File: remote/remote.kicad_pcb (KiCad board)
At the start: 2 copper layers, 0 parts

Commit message: devlog 04
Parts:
- added C1: 100nF, Capacitor_SMD:C_0603_1608Metric, F.Cu at (0.00, 0.00)
- added C2: 10uF, Capacitor_SMD:C_0603_1608Metric, F.Cu at (0.00, 0.00)
- added C3: 1uF, Capacitor_SMD:C_0603_1608Metric, F.Cu at (0.00, 0.00)
- added D_CHG: CHG, LED_SMD:LED_0603_1608Metric, F.Cu at (0.00, 0.00)
- added D_STAT: STATUS, LED_SMD:LED_0603_1608Metric, F.Cu at (0.00, 0.00)
- added D_VBAT, D_VBUS: SS14, Diode_SMD:D_SMA, F.Cu at (0.00, 0.00)
- added HDR1: DEBUG, Connector_PinHeader_2.54mm:PinHeader_1x03_P2.54mm_Vertical, F.Cu at (0.00, 0.00)
- added J1: USB-C, Connector_USB:USB_C_Receptacle_HRO_TYPE-C-31-M-12, F.Cu at (0.00, 0.00)
- added J_BAT: BAT, Connector_JST:JST_PH_B2B-PH-K_1x02_P2.00mm_Vertical, F.Cu at (0.00, 0.00)
- added R_CC1, R_CC2: 5.1k, Resistor_SMD:R_0603_1608Metric, F.Cu at (0.00, 0.00)
- added R_CHG, R_STAT: 1k, Resistor_SMD:R_0603_1608Metric, F.Cu at (0.00, 0.00)
- added R_DN, R_UP: 100k, Resistor_SMD:R_0603_1608Metric, F.Cu at (0.00, 0.00)
- added R_EN: 10k, Resistor_SMD:R_0603_1608Metric, F.Cu at (0.00, 0.00)
- added R_PROG: 2k, Resistor_SMD:R_0603_1608Metric, F.Cu at (0.00, 0.00)
- added SW1: Choc1, clicker:Choc_V1_PG1350, F.Cu at (0.00, 0.00)
- added SW2: Choc2, clicker:Choc_V1_PG1350, F.Cu at (0.00, 0.00)
- added SW_BOOT: BOOT, Button_Switch_SMD:SW_SPST_B3U-1000P, F.Cu at (0.00, 0.00)
- added SW_PWR: POWER, Button_Switch_THT:SW_Slide_SPDT_Straight_CK_OS102011MS2Q, F.Cu at (0.00, 0.00)
- added SW_RST: RESET, Button_Switch_SMD:SW_SPST_B3U-1000P, F.Cu at (0.00, 0.00)
- added U1: ESP32-C3-WROOM-02, RF_Module:ESP32-C3-WROOM-02, F.Cu at (0.00, 0.00)
- added U2: MCP73831, Package_TO_SOT_SMD:SOT-23-5, F.Cu at (0.00, 0.00)
- added U3: AP2112K-3.3, Package_TO_SOT_SMD:SOT-23-5, F.Cu at (0.00, 0.00)

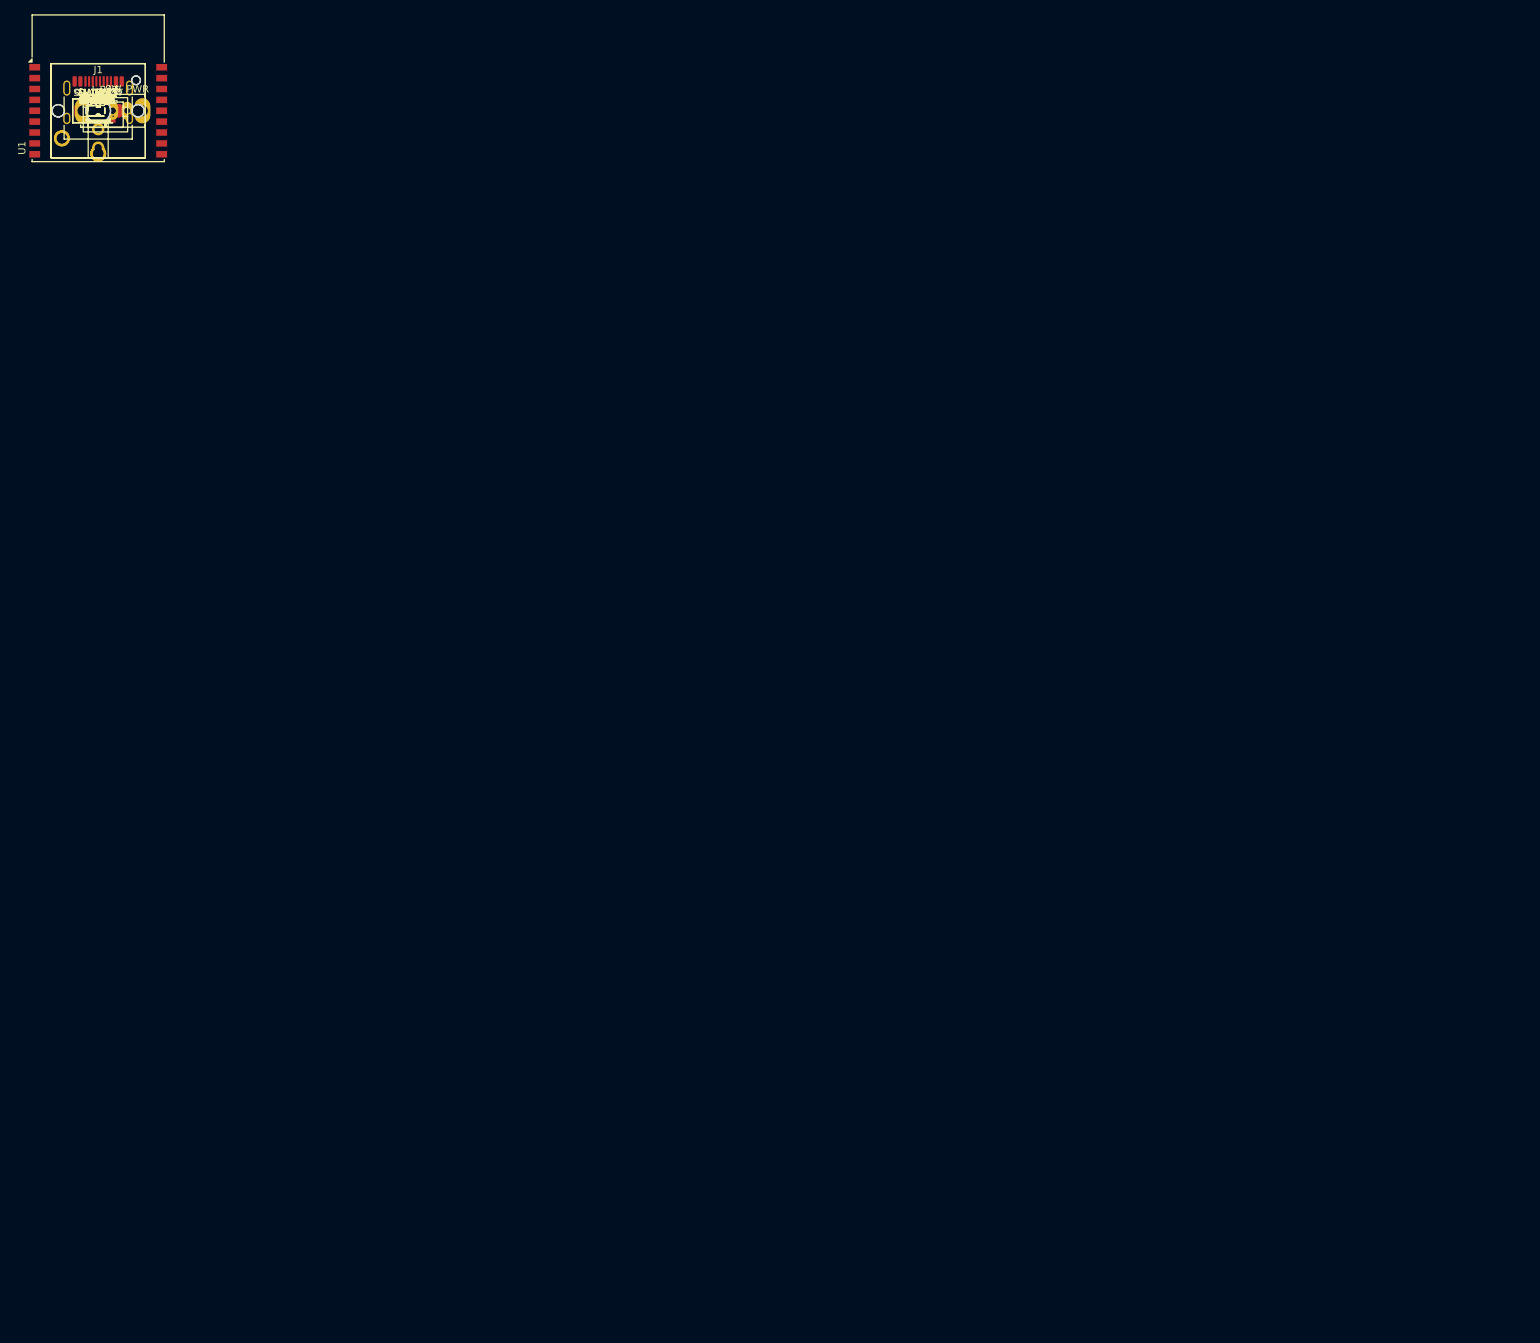
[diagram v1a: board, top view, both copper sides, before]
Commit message: devlog 06
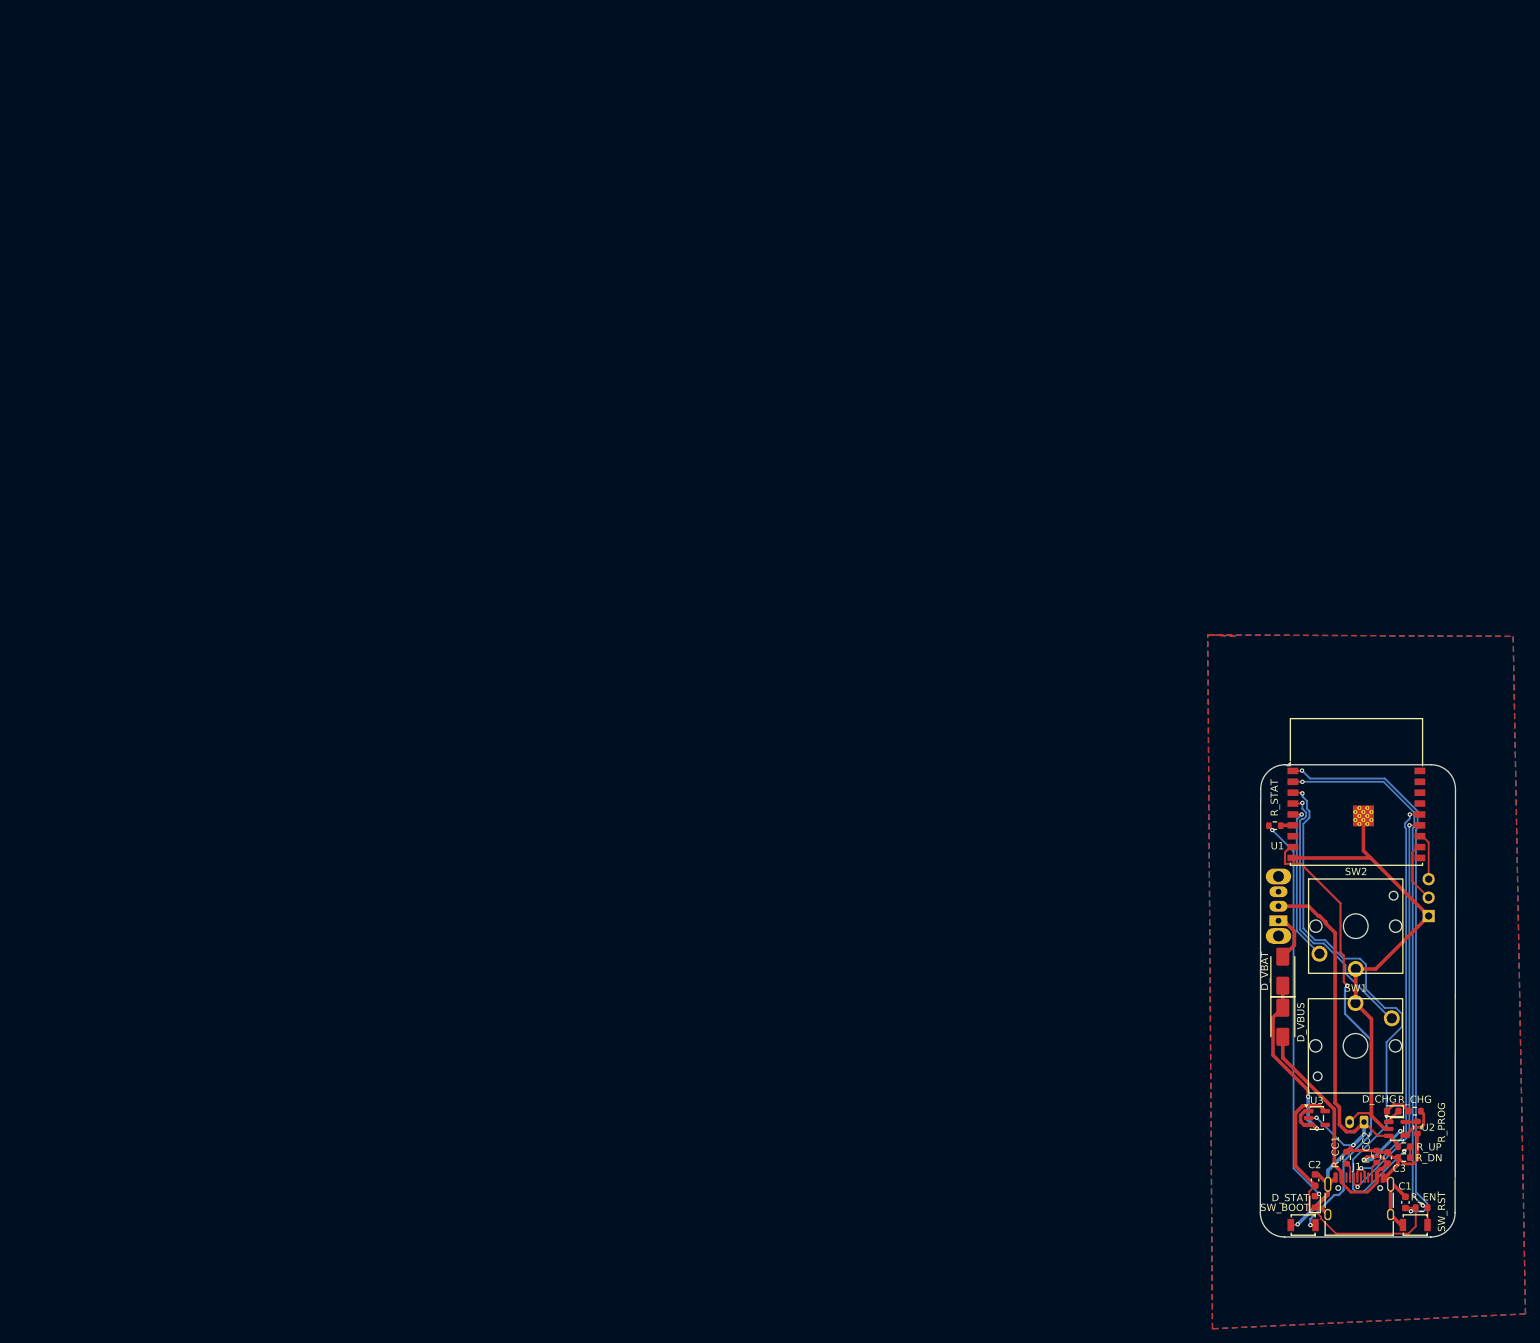
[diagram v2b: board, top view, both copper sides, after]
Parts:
- HDR1, J_BAT, SW_PWR: moved to B.Cu
- moved SW_RST 237.8 mm to (181.6, 153.6)
- moved R_EN 237.0 mm to (182.4, 151.2), turned to 180 degrees
- moved C1 234.8 mm to (180.2, 150.5), turned to 90 degrees
- moved R_DN 230.7 mm to (180.0, 144.3), turned to 180 degrees
- moved J1 230.3 mm to (173.8, 151.1)
- moved R_UP 229.8 mm to (180.0, 142.8)
- moved R_PROG 229.6 mm to (181.8, 140.2), turned to -90 degrees
- moved C3 229.0 mm to (177.8, 144.3), turned to 90 degrees
- moved R_CHG 227.9 mm to (181.5, 137.9), turned to 180 degrees
- moved R_CC2 227.7 mm to (176.2, 144.2), turned to 90 degrees
- moved U2 227.5 mm to (179.0, 140.3)
- moved SW_BOOT 226.2 mm to (166.1, 153.6)
- moved D_CHG 225.5 mm to (178.4, 137.9), turned to 180 degrees
- moved D_STAT 225.3 mm to (167.8, 150.4), turned to 90 degrees
- moved R_CC1 224.6 mm to (172.1, 144.3), turned to 90 degrees
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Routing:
- net GND: track 0.00 -> 136.1 mm, vias 0 -> 3
- net 3v3: track 0.00 -> 118.5 mm, vias 0 -> 2
- net VSENSE: track 0.00 -> 80.2 mm, vias 0 -> 2
- net EN_NET: track 0.00 -> 76.5 mm, vias 0 -> 2
- net BOOT_NET: track 0.00 -> 63.8 mm, vias 0 -> 2
- net USB_DN: track 0.00 -> 57.3 mm, vias 0 -> 2
- net USB_DP: track 0.00 -> 57.0 mm, vias 0 -> 2
- net STAT_A: track 0.00 -> 54.3 mm, vias 0 -> 2
- net VBUS: track 0.00 -> 49.6 mm, vias 0 -> 2
- net BAT_P: track 0.00 -> 46.7 mm
- net SW1_NET: track 0.00 -> 37.9 mm, vias 0 -> 1
- net VSYS: track 0.00 -> 27.7 mm, vias 0 -> 2
- net SW2_NET: track 0.00 -> 22.0 mm, vias 0 -> 1
- net UART_RX: track 0.00 -> 8.52 mm
- net VBAT_SYS: track 0.00 -> 6.96 mm
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- added copper zone on B.Cu, net GND
- added copper zone on F.Cu, net GND
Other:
- board outline added: 26.9 x 65.1 mm

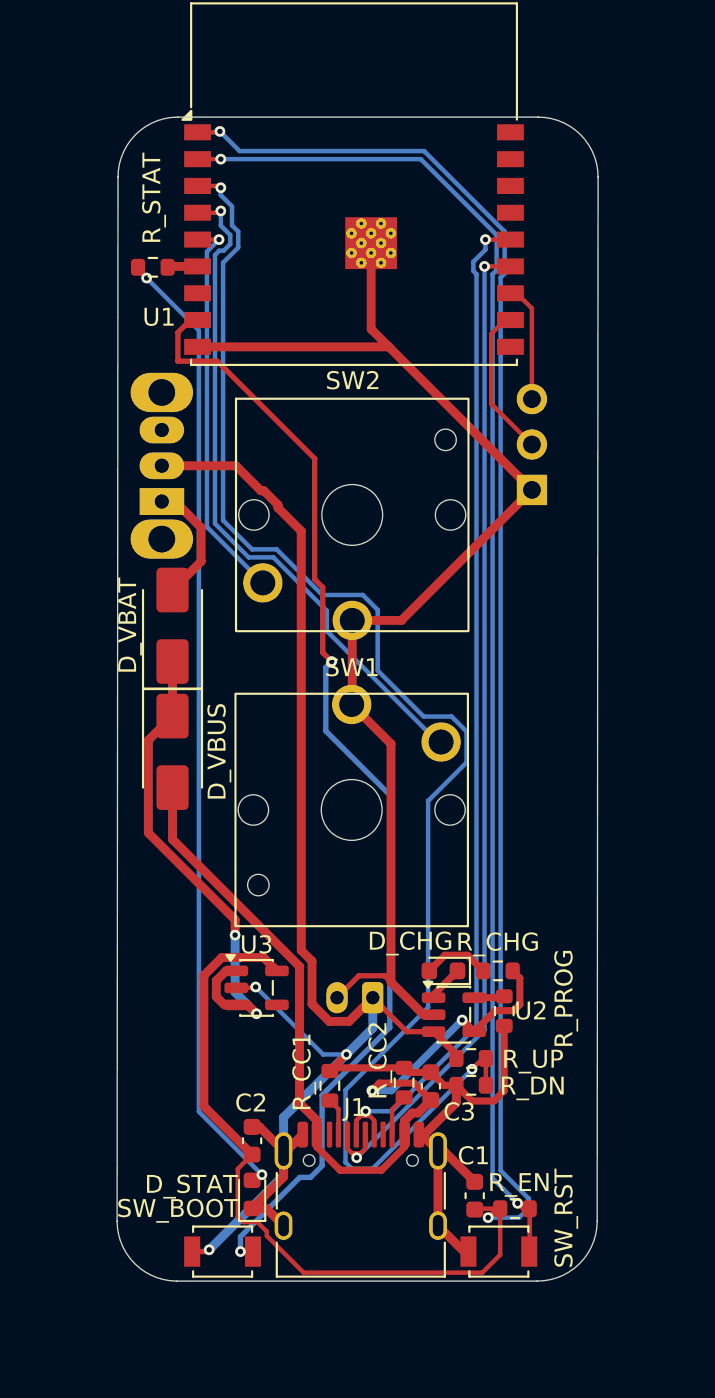
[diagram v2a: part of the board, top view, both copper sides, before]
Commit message: devlog 07
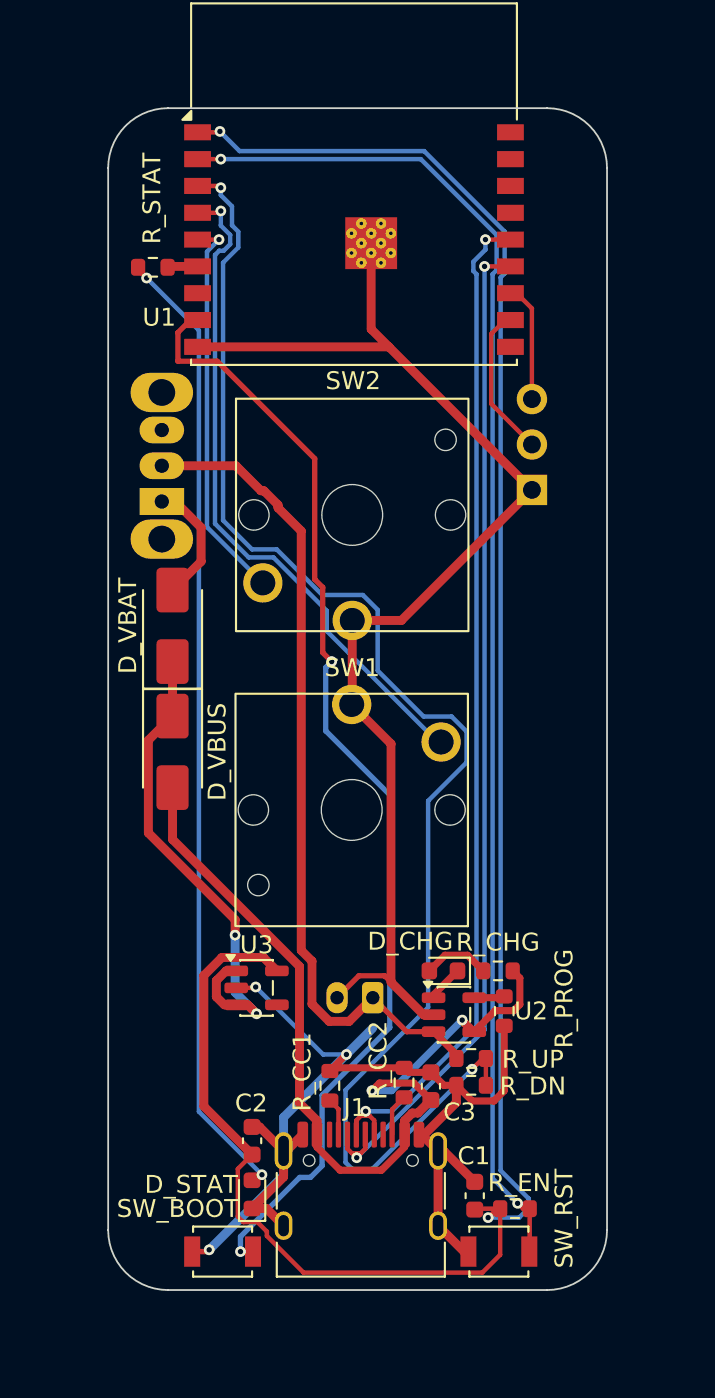
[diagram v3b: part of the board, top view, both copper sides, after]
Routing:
- net GND: track 136.1 -> 134.3 mm
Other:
- board size 26.9 x 65.1 mm -> 27.9 x 66.1 mm
